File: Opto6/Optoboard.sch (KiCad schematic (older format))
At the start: 50 parts, among them J1 S1 Connector, J2 S2 Connector, J3 S3 Connector, J4 S4 Connector, J6 S5 Connector, J7 S6 Connector, P1 CONN_01X08, U1 6N135, U2 6N135, U3 6N135, U4 6N135, U5 6N135, U6 6N135, U7 L7805

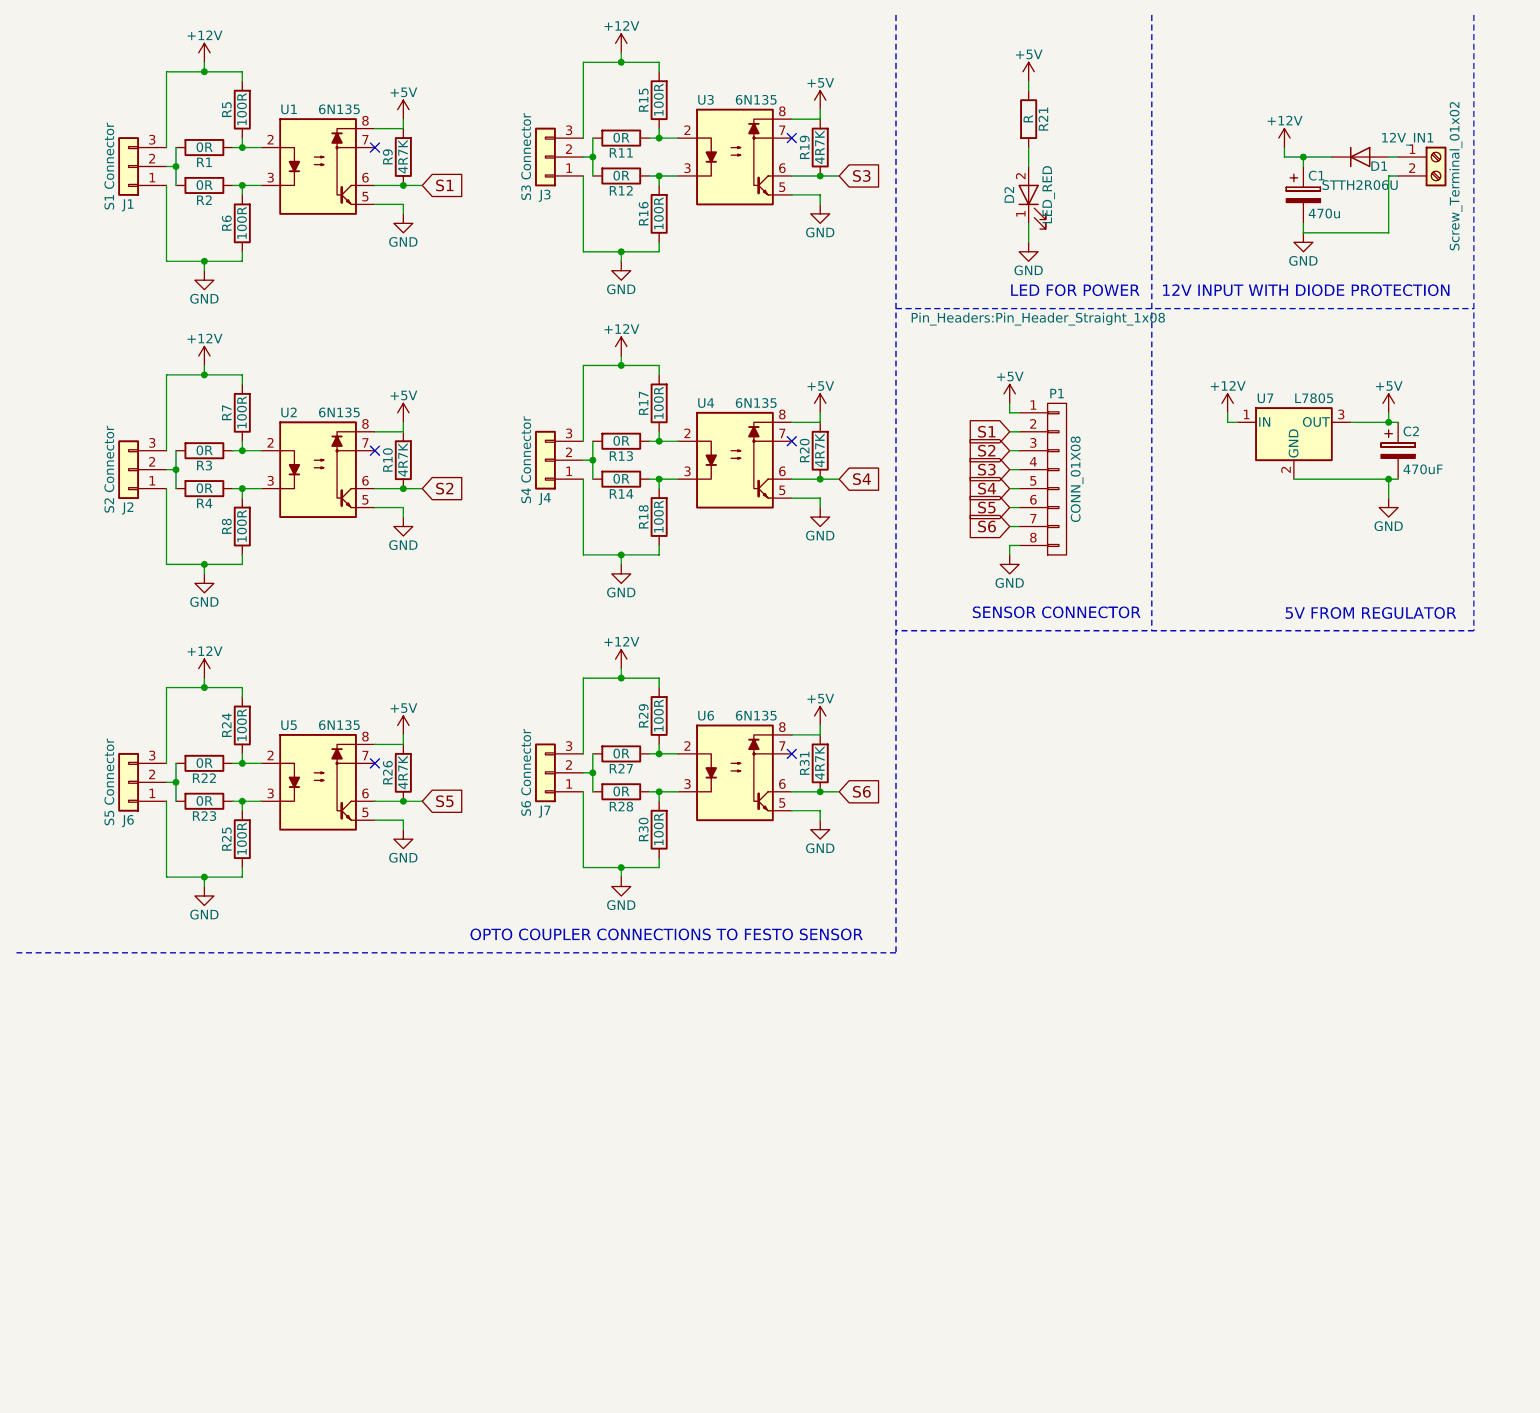
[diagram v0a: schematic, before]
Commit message: Added files
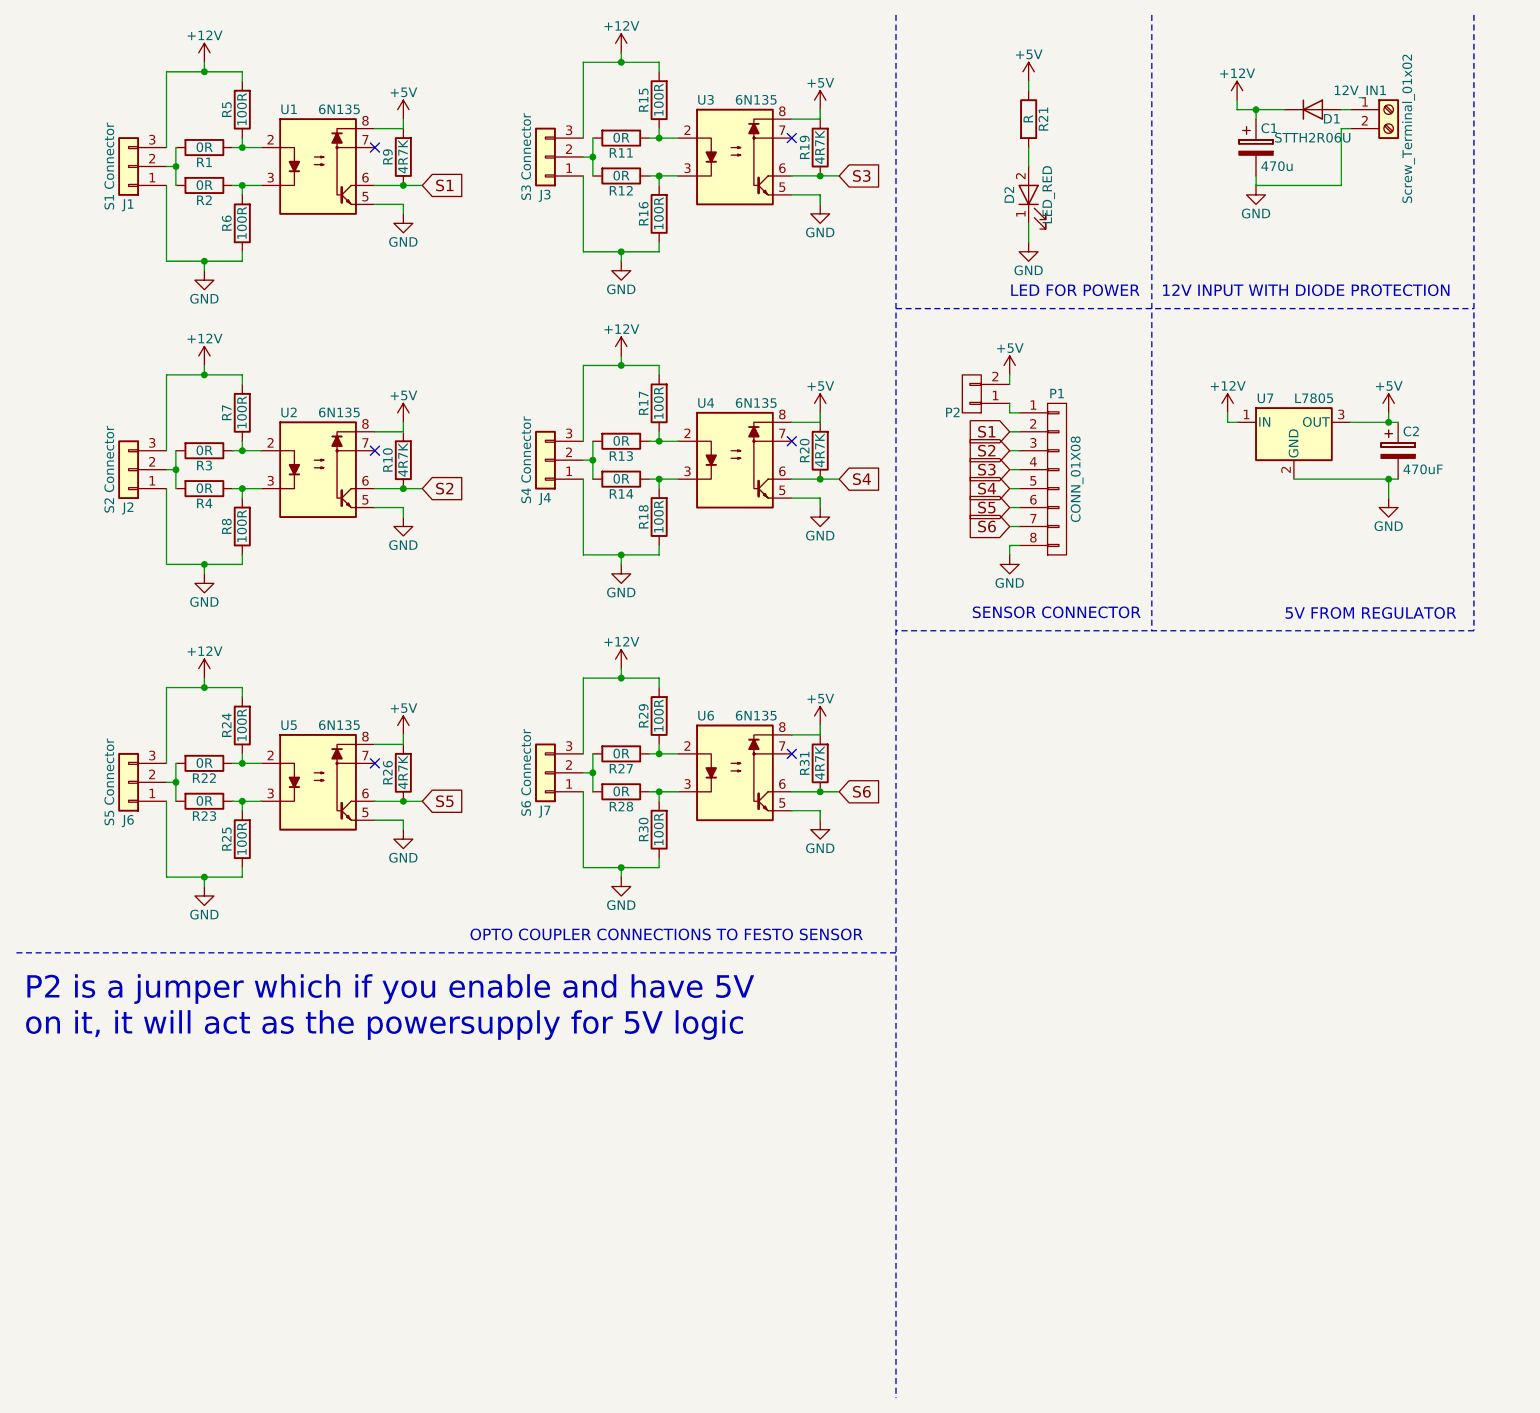
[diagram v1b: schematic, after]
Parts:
- added P2: CONN_01X02, Pin_Headers:Pin_Header_Straight_1x02, symbol CONN_01X02
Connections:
- net +5V: now also P2.2 (P2); no longer P1.1 (P1)
- new net: P1.1 (P1), P2.1 (P1)
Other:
- note added: "P2 is a jumper which if you enable and have 5V \non it, it will act as the powersupply for 5V logic"
- moved on the sheet: 12V_IN1, C1, D1
